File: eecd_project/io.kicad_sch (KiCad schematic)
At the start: 39 parts, among them J2 Screw_Terminal_01x04, J3 Screw_Terminal_01x03, J4 Screw_Terminal_01x03, J5 Screw_Terminal_01x03, J6 Screw_Terminal_01x03, K1 PE014024, K2 PE014024, K3 PE014024, K4 PE014024, Q5 MMBT3904, Q6 MMBT3904, Q7 MMBT3904, Q8 MMBT3904, U3 LTV-844, U4 LTV-844

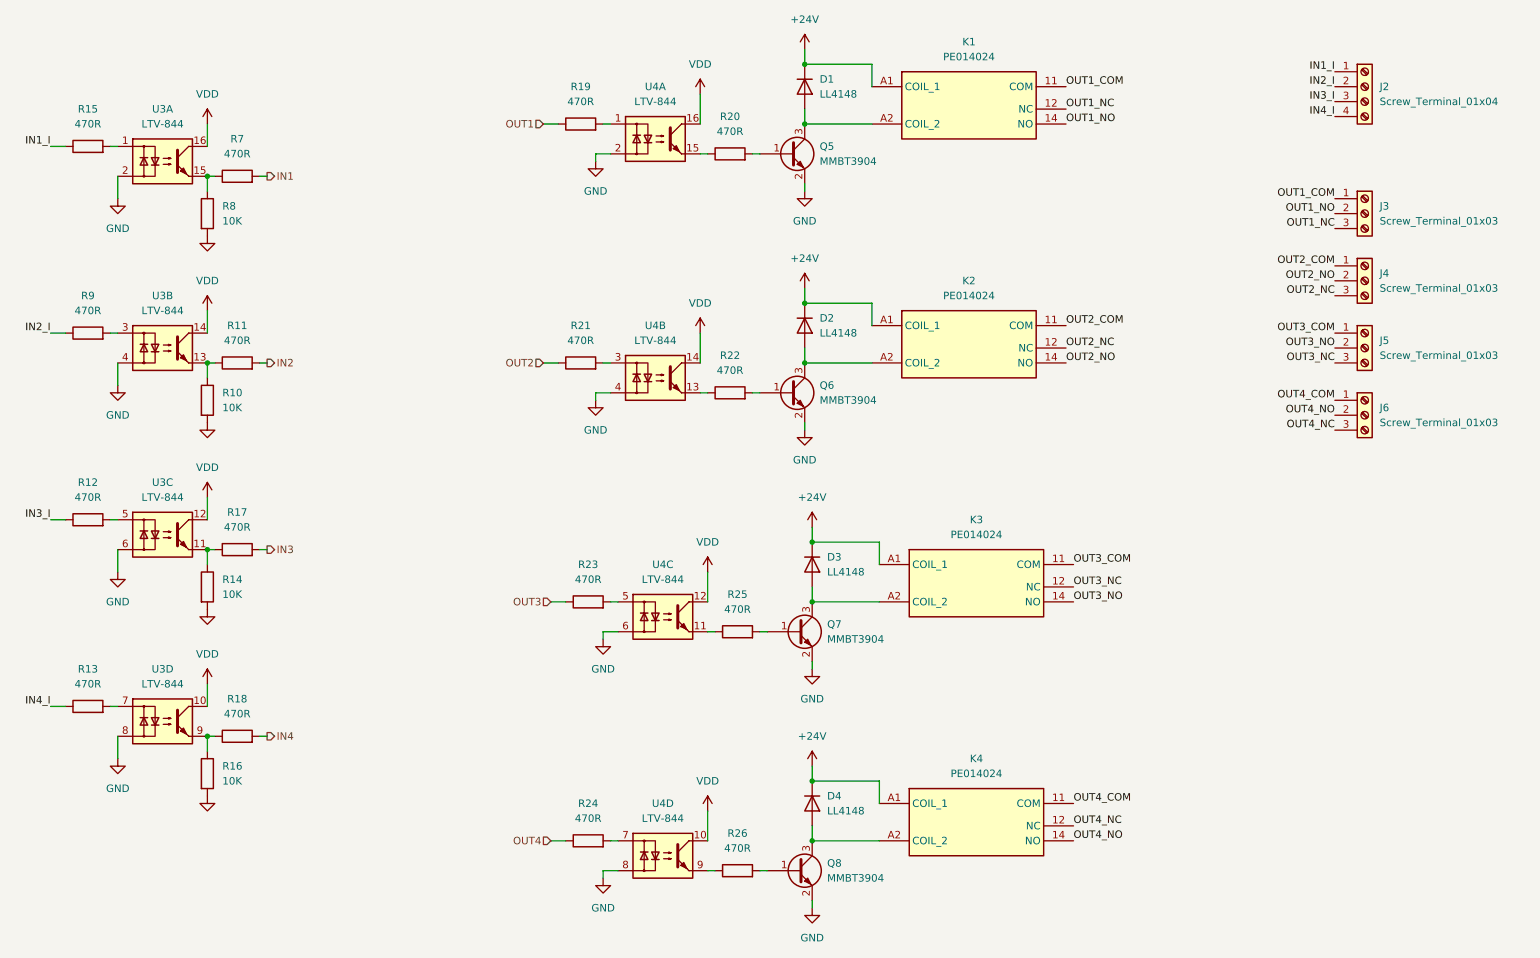
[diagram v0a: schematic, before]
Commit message: v3
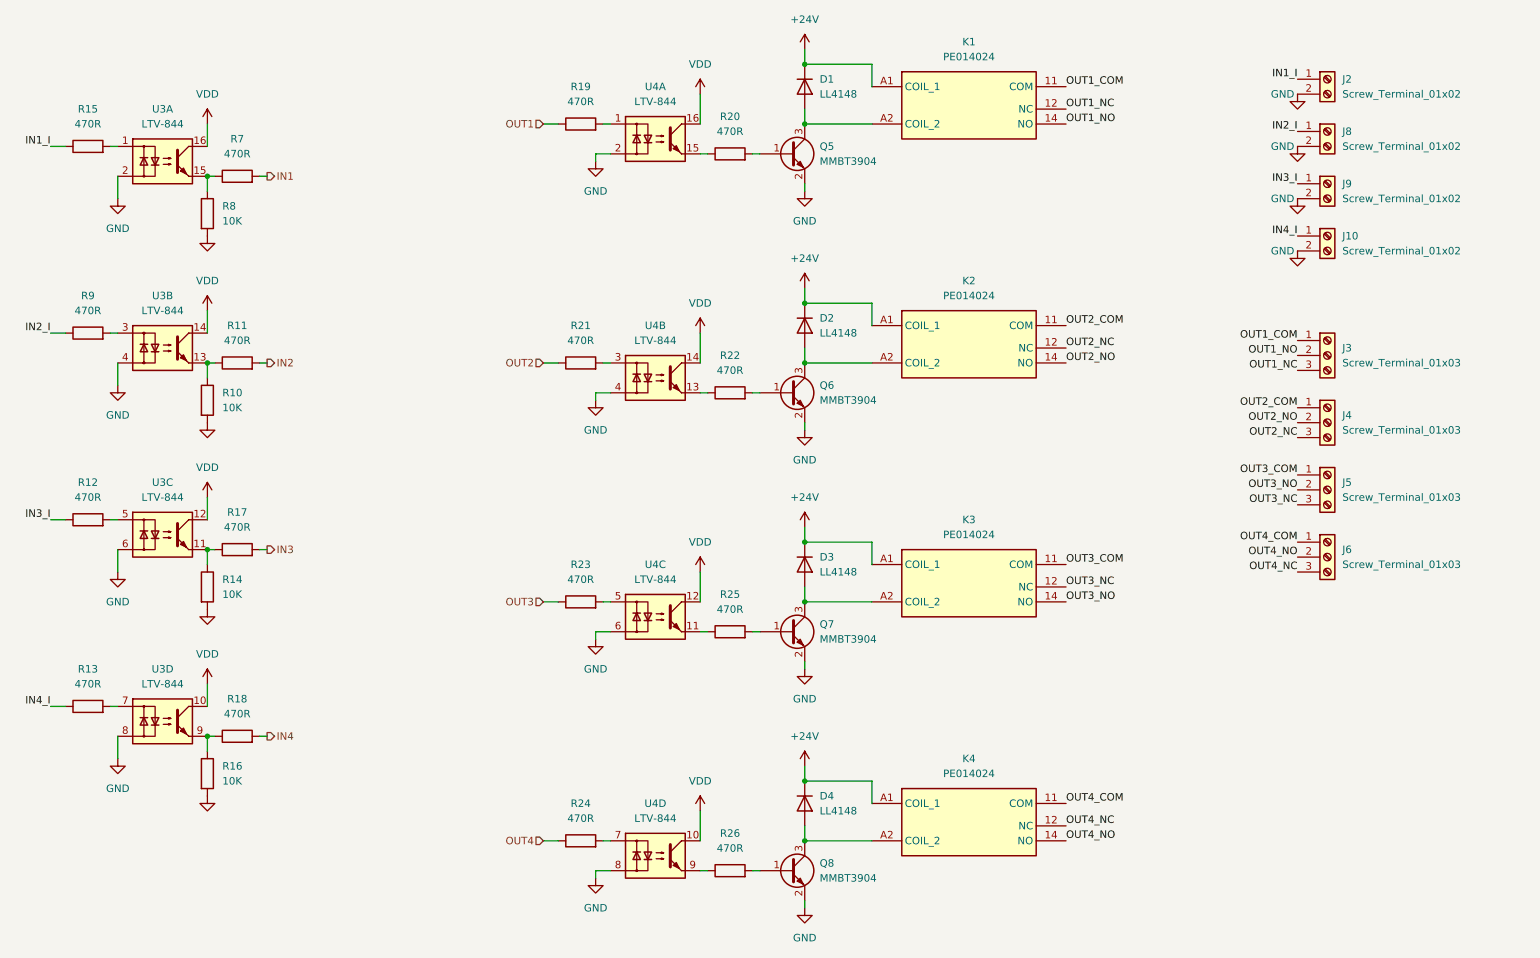
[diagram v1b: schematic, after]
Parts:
- removed J2: Screw_Terminal_01x04, symbol Connector:Screw_Terminal_01x04
- added J10, J2, J8, J9: Screw_Terminal_01x02, symbol Connector:Screw_Terminal_01x02
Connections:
- net GND: now also J10.2 (Pin_2), J2.2 (Pin_2), J8.2 (Pin_2), J9.2 (Pin_2)
- net IN1_I: now also J2.1 (Pin_1)
- net IN2_I: now also J8.1 (Pin_1)
- net IN3_I: now also J9.1 (Pin_1)
- net IN4_I: now also J10.1 (Pin_1)
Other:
- moved on the sheet: D3, D4, J3, J4, J5, J6, K3, K4, Q7, Q8, R23, R24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
